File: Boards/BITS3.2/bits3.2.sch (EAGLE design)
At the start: 32 parts, among them U1 LMR16020, X2 53398-10

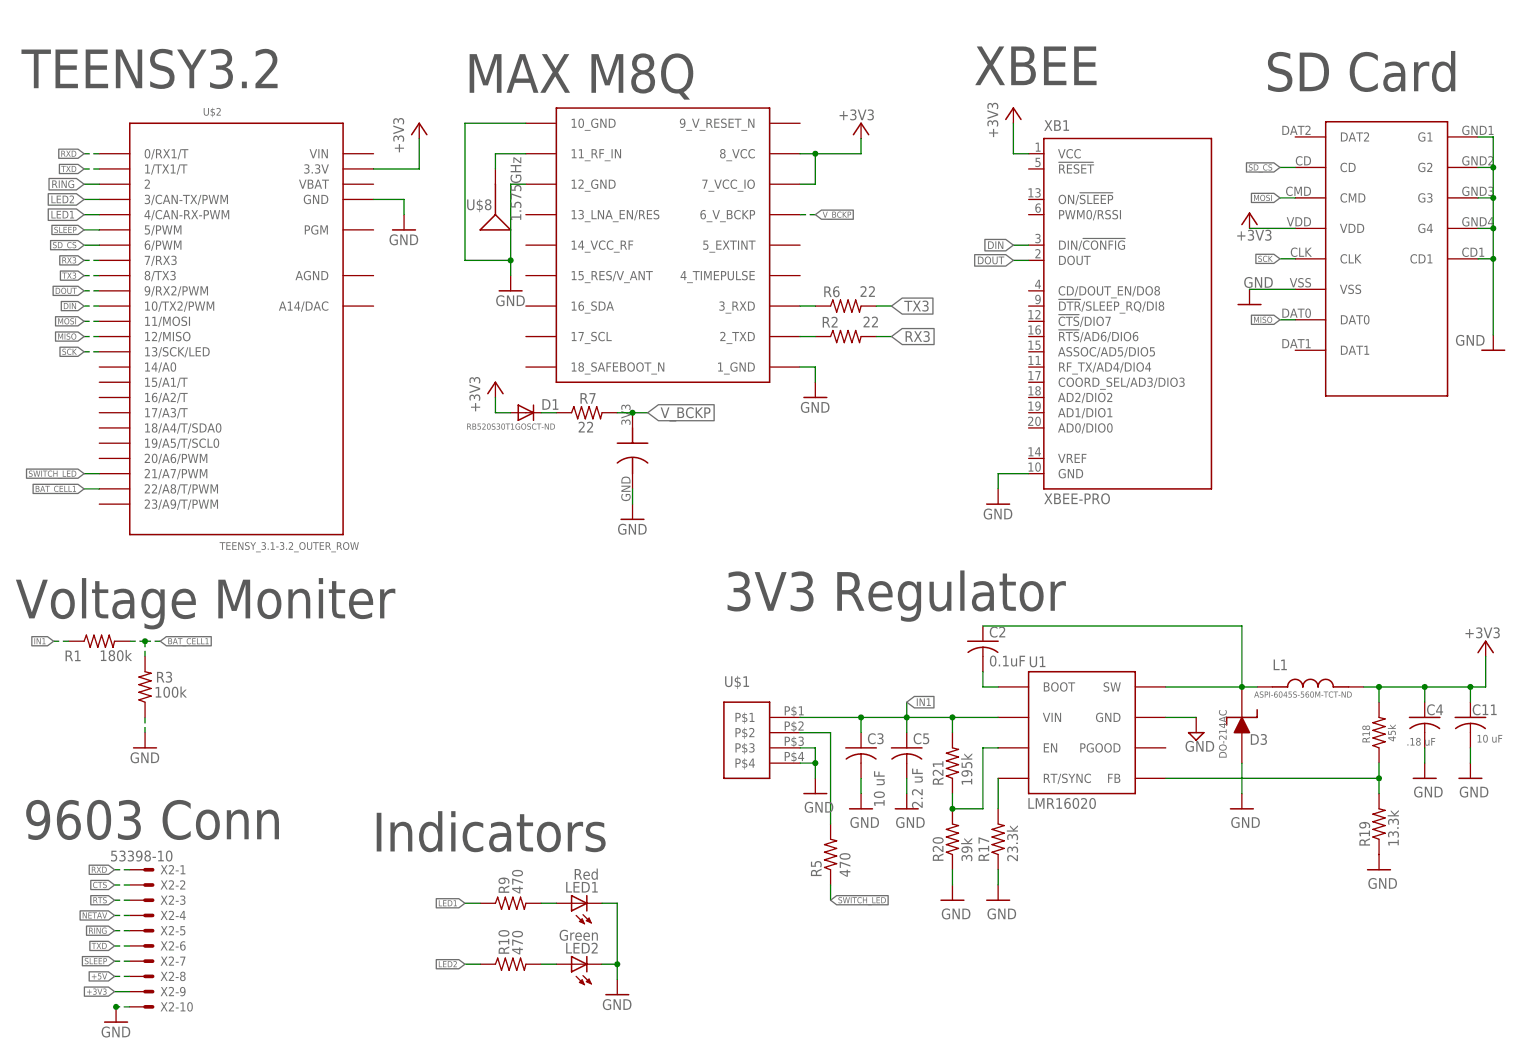
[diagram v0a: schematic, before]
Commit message: More stuff, close, not done
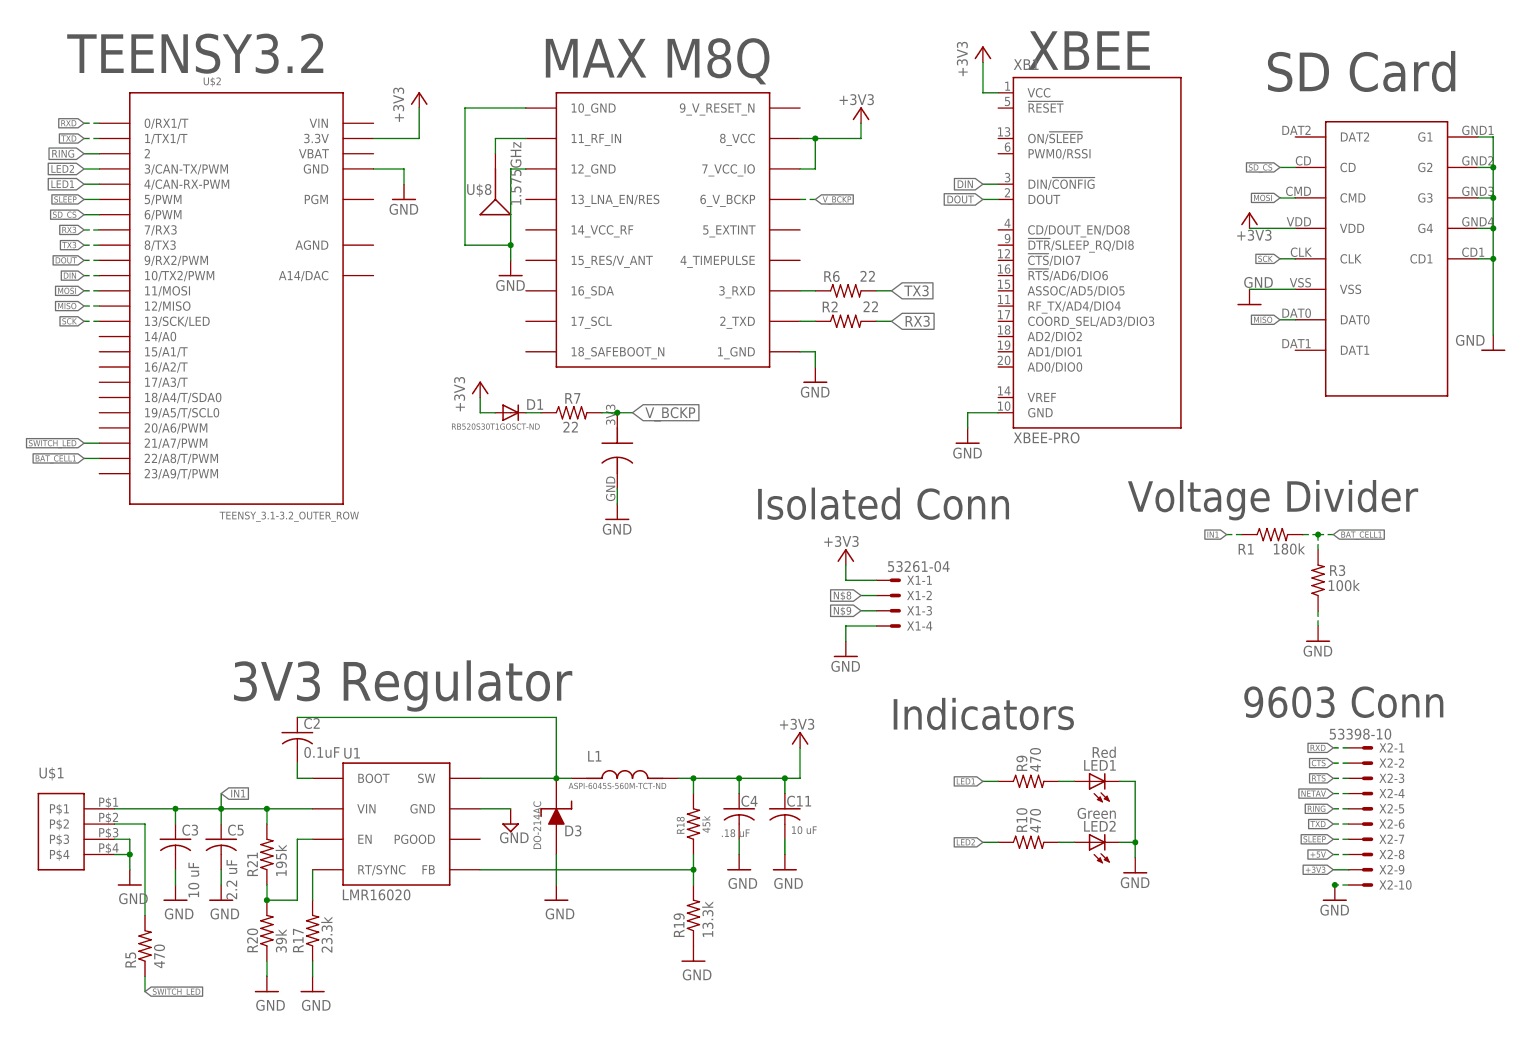
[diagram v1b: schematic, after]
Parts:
- added X1: 53261-04, con-molex:53261-04
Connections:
- new net N$8: X1-2.S
- new net N$9: X1-3.S
- net +3V3: now also X1-1.S
- net GND: now also X1-4.S
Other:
- note added: "Isolated Conn"
- note added: "Voltage Divider"
- note removed: "Voltage Moniter"
- moved on the sheet: C11, C2, C3, C4, C5, D1, D3, L1, LED1, LED2, R1, R10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
